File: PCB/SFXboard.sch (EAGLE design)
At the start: 19 parts, among them J1 AVR_SPI_PRG_6PTH, J2 TERMBLOCK4POS, J3 POWER_JACKPTH, Q1 16MHz, Q2 BSS138, Q3 BSS138, Q4 BSS138, U1 ATMEGA16U2-AU, X1 USBSMD

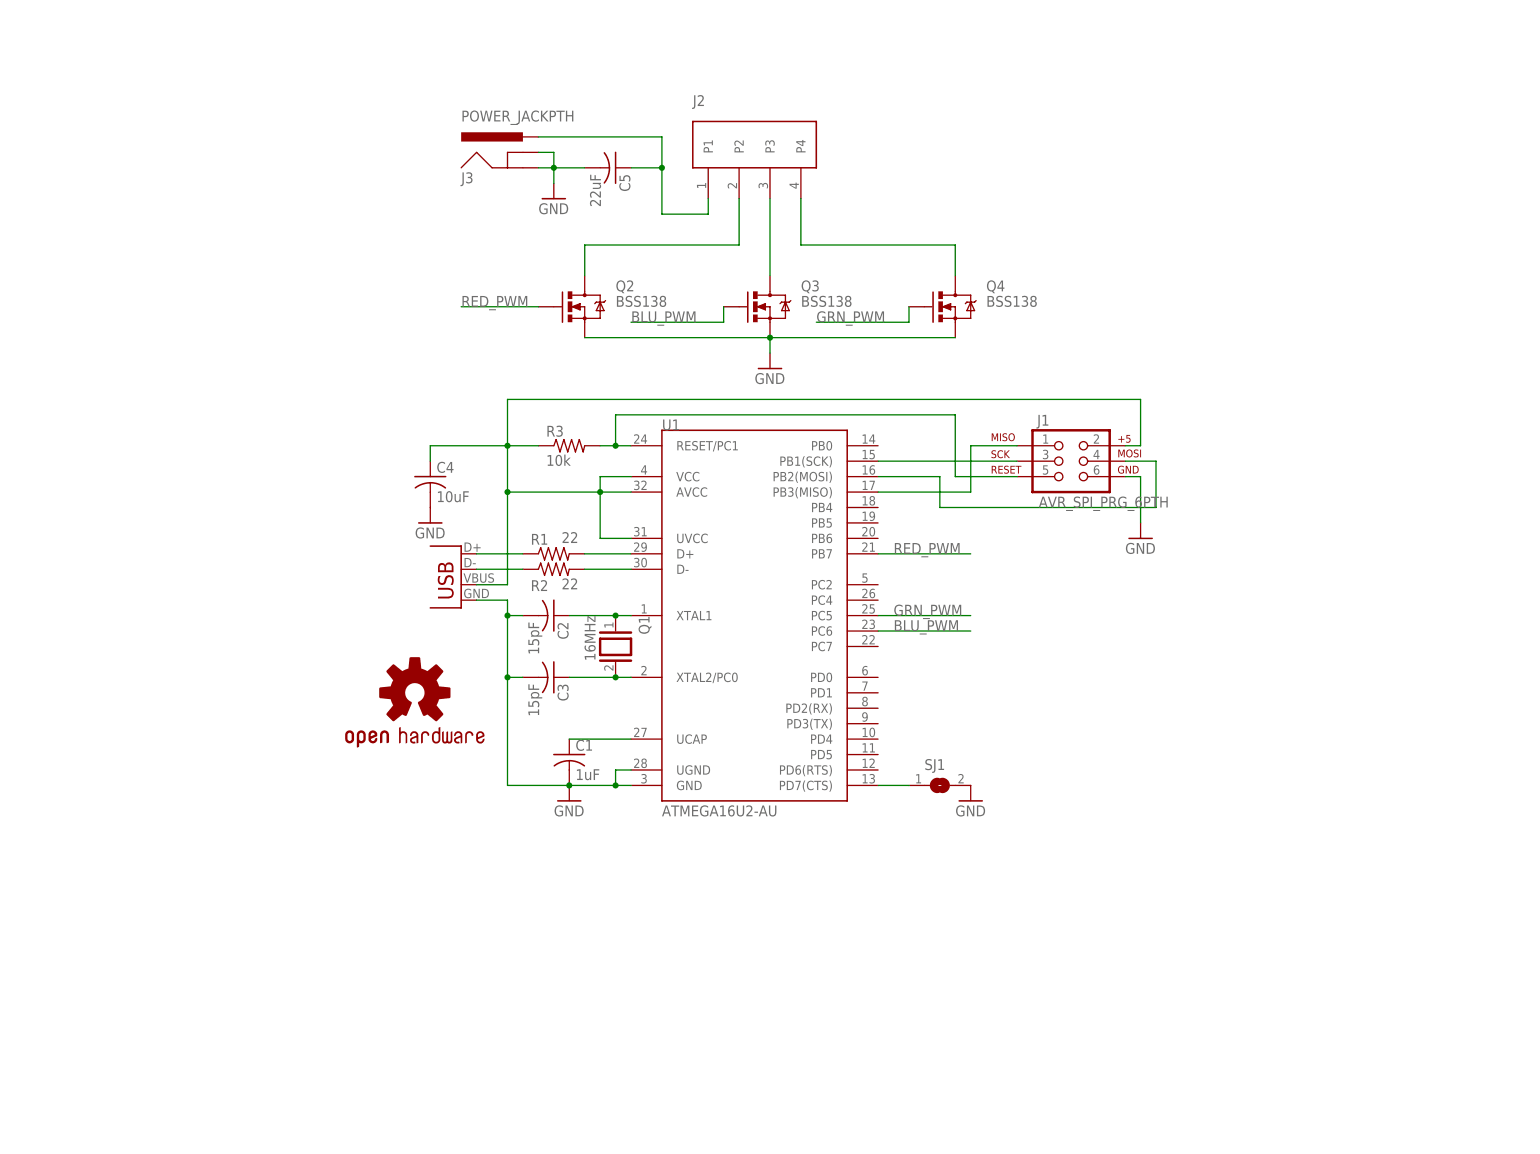
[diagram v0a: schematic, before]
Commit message: Circuit improvements, but not yet complete
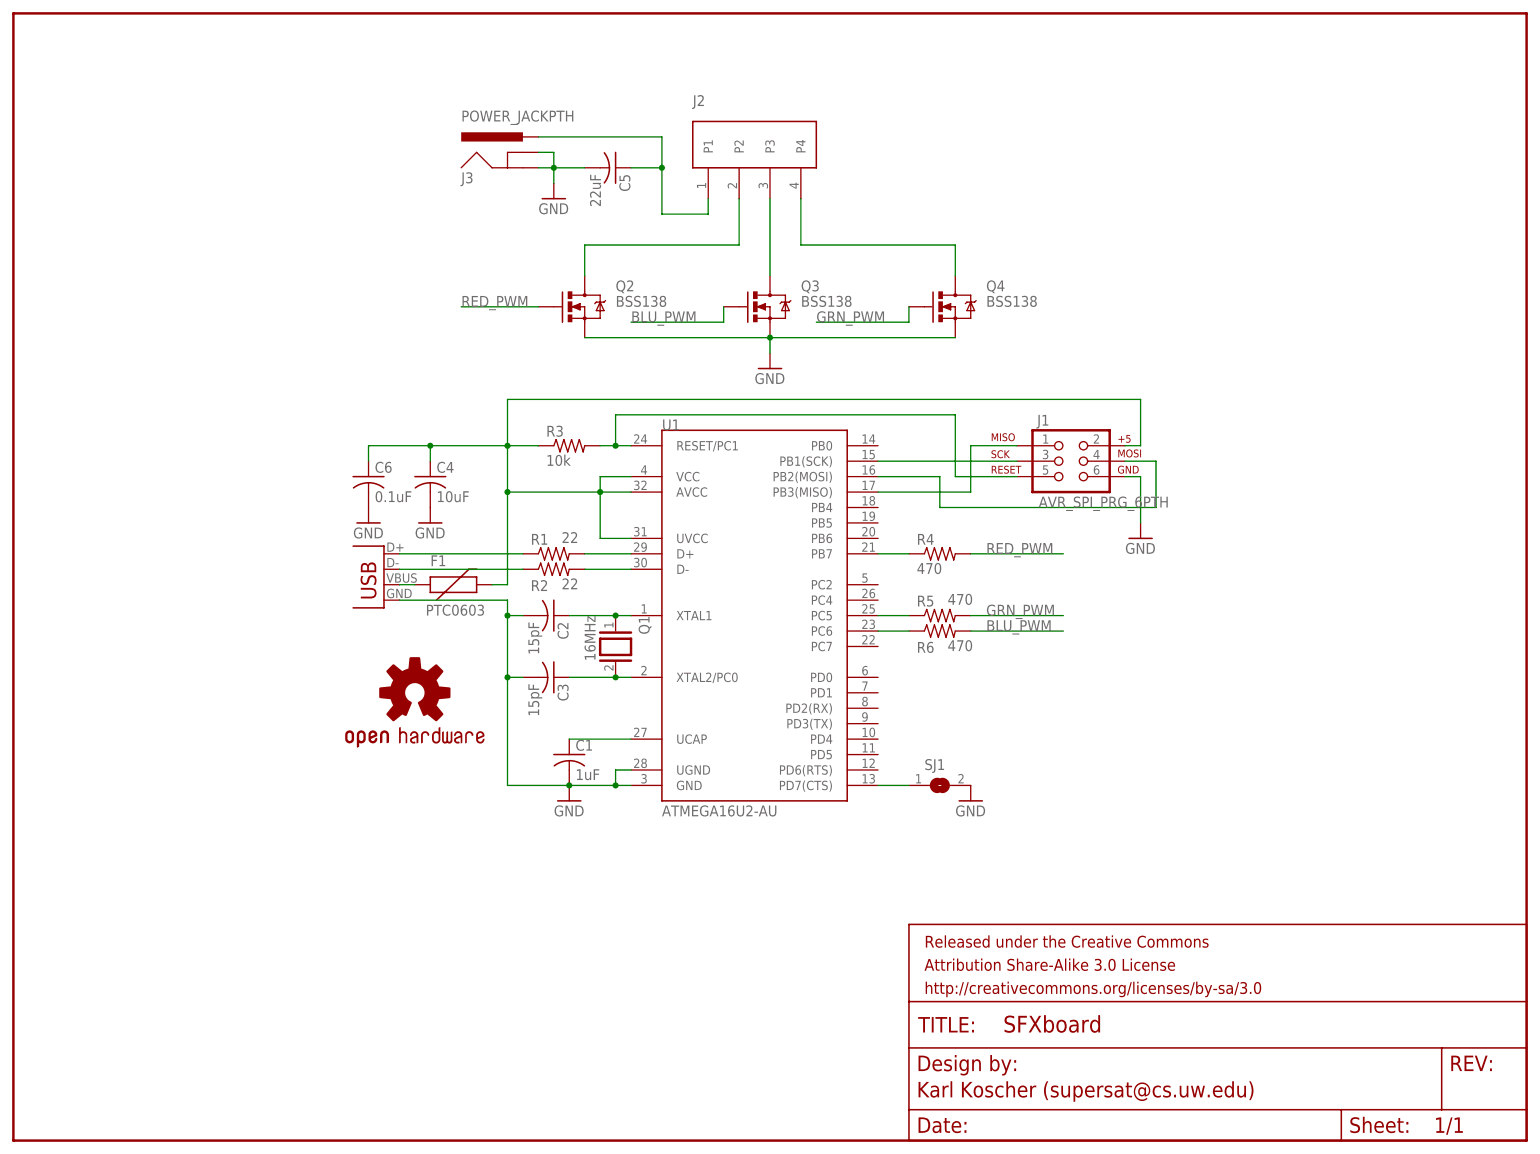
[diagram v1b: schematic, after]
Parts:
- added C6: 0.1uF, resistor:C-USC0402
- added F1: PTC0603, SparkFun-PowerIC:PTC0603
- added FRAME1: FRAME-LETTER, SparkFun-Aesthetics:FRAME-LETTER
- added R4, R5, R6: 470, resistor:R-US_R0805
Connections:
- new net B: R6.1, U1.PC6
- new net G: R5.1, U1.PC5
- new net N$18: C4.1, C6.1, F1.2, J1.2, R3.1, U1.AVCC, U1.UVCC, U1.VCC
- new net R: R4.1, U1.PB7
- net BLU_PWM: now also R6.2; no longer U1.PC6
- net GND: now also C6.2
- net GRN_PWM: now also R5.2; no longer U1.PC5
- net N$2: now also F1.1; no longer C4.1, J1.2, R3.1, U1.AVCC, U1.UVCC, U1.VCC
- net RED_PWM: now also R4.2; no longer U1.PB7
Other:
- note added: "Karl Koscher (supersat@cs.uw.edu)"
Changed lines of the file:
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@@
 <part name="SJ1" library="jumper" deviceset="SJ" device=""/>
 <part name="GND6" library="supply1" deviceset="GND" device=""/>
+<part name="C6" library="resistor" deviceset="C-US" device="C0402" value="0.1uF"/>
+<part name="GND7" library="supply1" deviceset="GND" device=""/>
+<part name="R4" library="resistor" deviceset="R-US_" device="R0805" value="470"/>
+<part name="R5" library="resistor" deviceset="R-US_" device="R0805" value="470"/>
+<part name="R6" library="resistor" deviceset="R-US_" device="R0805" value="470"/>
+<part name="FRAME1" library="SparkFun-Aesthetics" deviceset="FRAME-LETTER" device=""/>
+<part name="F1" library="SparkFun-PowerIC" deviceset="PTC" device="0603"/>
 </parts>
 <sheets>
 <sheet>
 <plain>
+<text x="26.67" y="-79.248" size="2.54" layer="94">Karl Koscher (supersat@cs.uw.edu)</text>
 </plain>
 <instances>
@@
 <instance part="C1" gate="G$1" x="-30.48" y="-22.86"/>
 <instance part="GND1" gate="1" x="-30.48" y="-30.48"/>
-<instance part="X1" gate="G$1" x="-48.26" y="2.54" rot="MR0"/>
+<instance part="X1" gate="G$1" x="-60.96" y="2.54" rot="MR0"/>
 <instance part="R1" gate="G$1" x="-33.02" y="10.16" smashed="yes">
 <attribute name="NAME" x="-36.83" y="11.6586" size="1.778" layer="95"/>
@@
 <instance part="SJ1" gate="1" x="30.48" y="-27.94"/>
 <instance part="GND6" gate="1" x="35.56" y="-30.48"/>
+<instance part="C6" gate="G$1" x="-63.5" y="22.86"/>
+<instance part="GND7" gate="1" x="-63.5" y="15.24"/>
+<instance part="R4" gate="G$1" x="30.48" y="10.16"/>
+<instance part="R5" gate="G$1" x="30.48" y="0" smashed="yes">
+<attribute name="NAME" x="26.67" y="1.4986" size="1.778" layer="95"/>
+<attribute name="VALUE" x="31.75" y="1.778" size="1.778" layer="96"/>
+</instance>
+<instance part="R6" gate="G$1" x="30.48" y="-2.54" smashed="yes">
+<attribute name="NAME" x="26.67" y="-6.1214" size="1.778" layer="95"/>
+<attribute name="VALUE" x="31.75" y="-5.842" size="1.778" layer="96"/>
+</instance>
+<instance part="FRAME1" gate="G$1" x="-121.92" y="-86.36"/>
+<instance part="FRAME1" gate="G$2" x="25.4" y="-86.36"/>
+<instance part="F1" gate="G$1" x="-50.8" y="5.08"/>
 </instances>
 <busses>
@@
 <wire x1="-40.64" y1="-10.16" x2="-40.64" y2="0" width="0.1524" layer="91"/>
 <wire x1="-40.64" y1="0" x2="-40.64" y2="2.54" width="0.1524" layer="91"/>
-<wire x1="-40.64" y1="2.54" x2="-45.72" y2="2.54" width="0.1524" layer="91"/>
+<wire x1="-40.64" y1="2.54" x2="-58.42" y2="2.54" width="0.1524" layer="91"/>
 <pinref part="C2" gate="G$1" pin="2"/>
 <wire x1="-38.1" y1="0" x2="-40.64" y2="0" width="0.1524" layer="91"/>
@@
 <pinref part="GND6" gate="1" pin="GND"/>
 </segment>
-</net>
-<net name="N$2" class="0">
-<segment>
-<pinref part="U1" gate="G$1" pin="VCC"/>
-<wire x1="-20.32" y1="22.86" x2="-25.4" y2="22.86" width="0.1524" layer="91"/>
-<wire x1="-25.4" y1="22.86" x2="-25.4" y2="20.32" width="0.1524" layer="91"/>
-<pinref part="U1" gate="G$1" pin="AVCC"/>
-<wire x1="-25.4" y1="20.32" x2="-20.32" y2="20.32" width="0.1524" layer="91"/>
-<pinref part="U1" gate="G$1" pin="UVCC"/>
-<wire x1="-20.32" y1="12.7" x2="-25.4" y2="12.7" width="0.1524" layer="91"/>
-<wire x1="-25.4" y1="20.32" x2="-25.4" y2="12.7" width="0.1524" layer="91"/>
-<pinref part="X1" gate="G$1" pin="VBUS"/>
-<wire x1="-45.72" y1="5.08" x2="-40.64" y2="5.08" width="0.1524" layer="91"/>
-<wire x1="-40.64" y1="5.08" x2="-40.64" y2="20.32" width="0.1524" layer="91"/>
-<wire x1="-40.64" y1="20.32" x2="-25.4" y2="20.32" width="0.1524" layer="91"/>
-<junction x="-25.4" y="20.32"/>
-<pinref part="R3" gate="G$1" pin="1"/>
-<wire x1="-35.56" y1="27.94" x2="-40.64" y2="27.94" width="0.1524" layer="91"/>
-<wire x1="-40.64" y1="27.94" x2="-40.64" y2="20.32" width="0.1524" layer="91"/>
-<junction x="-40.64" y="20.32"/>
-<pinref part="C4" gate="G$1" pin="1"/>
-<wire x1="-53.34" y1="25.4" x2="-53.34" y2="27.94" width="0.1524" layer="91"/>
-<wire x1="-53.34" y1="27.94" x2="-40.64" y2="27.94" width="0.1524" layer="91"/>
-<junction x="-40.64" y="27.94"/>
-<pinref part="J1" gate="G$1" pin="2"/>
-<wire x1="60.96" y1="27.94" x2="63.5" y2="27.94" width="0.1524" layer="91"/>
-<wire x1="63.5" y1="27.94" x2="63.5" y2="35.56" width="0.1524" layer="91"/>
-<wire x1="63.5" y1="35.56" x2="-40.64" y2="35.56" width="0.1524" layer="91"/>
-<wire x1="-40.64" y1="35.56" x2="-40.64" y2="27.94" width="0.1524" layer="91"/>
+<segment>
+<pinref part="C6" gate="G$1" pin="2"/>
+<pinref part="GND7" gate="1" pin="GND"/>
 </segment>
 </net>
@@
 <pinref part="X1" gate="G$1" pin="D+"/>
 <pinref part="R1" gate="G$1" pin="1"/>
-<wire x1="-45.72" y1="10.16" x2="-38.1" y2="10.16" width="0.1524" layer="91"/>
+<wire x1="-58.42" y1="10.16" x2="-38.1" y2="10.16" width="0.1524" layer="91"/>
 </segment>
 </net>
@@
 <pinref part="X1" gate="G$1" pin="D-"/>
 <pinref part="R2" gate="G$1" pin="1"/>
-<wire x1="-45.72" y1="7.62" x2="-38.1" y2="7.62" width="0.1524" layer="91"/>
+<wire x1="-58.42" y1="7.62" x2="-38.1" y2="7.62" width="0.1524" layer="91"/>
 </segment>
 </net>
@@
 <net name="RED_PWM" class="0">
 <segment>
-<pinref part="U1" gate="G$1" pin="PB7"/>
-<wire x1="20.32" y1="10.16" x2="35.56" y2="10.16" width="0.1524" layer="91"/>
-<label x="22.86" y="10.16" size="1.778" layer="95"/>
-</segment>
-<segment>
 <pinref part="Q2" gate="G$1" pin="G"/>
 <wire x1="-35.56" y1="50.8" x2="-48.26" y2="50.8" width="0.1524" layer="91"/>
 <label x="-48.26" y="50.8" size="1.778" layer="95"/>
+</segment>
+<segment>
+<pinref part="R4" gate="G$1" pin="2"/>
+<wire x1="35.56" y1="10.16" x2="50.8" y2="10.16" width="0.1524" layer="91"/>
+<label x="38.1" y="10.16" size="1.778" layer="95"/>
 </segment>
 </net>
@@
 </segment>
 <segment>
-<pinref part="U1" gate="G$1" pin="PC6"/>
-<wire x1="20.32" y1="-2.54" x2="35.56" y2="-2.54" width="0.1524" layer="91"/>
-<label x="22.86" y="-2.54" size="1.778" layer="95"/>
+<pinref part="R6" gate="G$1" pin="2"/>
+<wire x1="35.56" y1="-2.54" x2="50.8" y2="-2.54" width="0.1524" layer="91"/>
+<label x="38.1" y="-2.54" size="1.778" layer="95"/>
 </segment>
 </net>
@@
 </segment>
 <segment>
-<pinref part="U1" gate="G$1" pin="PC5"/>
-<wire x1="20.32" y1="0" x2="35.56" y2="0" width="0.1524" layer="91"/>
-<label x="22.86" y="0" size="1.778" layer="95"/>
+<pinref part="R5" gate="G$1" pin="2"/>
+<wire x1="35.56" y1="0" x2="50.8" y2="0" width="0.1524" layer="91"/>
+<label x="38.1" y="0" size="1.778" layer="95"/>
 </segment>
 </net>
@@
 </segment>
 </net>
+<net name="R" class="0">
+<segment>
+<pinref part="U1" gate="G$1" pin="PB7"/>
+<wire x1="20.32" y1="10.16" x2="25.4" y2="10.16" width="0.1524" layer="91"/>
+<pinref part="R4" gate="G$1" pin="1"/>
+</segment>
+</net>
+<net name="G" class="0">
+<segment>
+<pinref part="U1" gate="G$1" pin="PC5"/>
+<wire x1="20.32" y1="0" x2="25.4" y2="0" width="0.1524" layer="91"/>
+<pinref part="R5" gate="G$1" pin="1"/>
+</segment>
+</net>
+<net name="B" class="0">
+<segment>
+<pinref part="U1" gate="G$1" pin="PC6"/>
+<wire x1="20.32" y1="-2.54" x2="25.4" y2="-2.54" width="0.1524" layer="91"/>
+<pinref part="R6" gate="G$1" pin="1"/>
+</segment>
+</net>
+<net name="N$18" class="0">
+<segment>
+<pinref part="U1" gate="G$1" pin="VCC"/>
+<wire x1="-20.32" y1="22.86" x2="-25.4" y2="22.86" width="0.1524" layer="91"/>
+<wire x1="-25.4" y1="22.86" x2="-25.4" y2="20.32" width="0.1524" layer="91"/>
+<pinref part="U1" gate="G$1" pin="AVCC"/>
+<wire x1="-25.4" y1="20.32" x2="-20.32" y2="20.32" width="0.1524" layer="91"/>
+<pinref part="U1" gate="G$1" pin="UVCC"/>
+<wire x1="-20.32" y1="12.7" x2="-25.4" y2="12.7" width="0.1524" layer="91"/>
+<wire x1="-25.4" y1="20.32" x2="-25.4" y2="12.7" width="0.1524" layer="91"/>
+<wire x1="-40.64" y1="20.32" x2="-25.4" y2="20.32" width="0.1524" layer="91"/>
+<junction x="-25.4" y="20.32"/>
+<pinref part="R3" gate="G$1" pin="1"/>
+<wire x1="-35.56" y1="27.94" x2="-40.64" y2="27.94" width="0.1524" layer="91"/>
+<wire x1="-40.64" y1="27.94" x2="-40.64" y2="20.32" width="0.1524" layer="91"/>
+<pinref part="C4" gate="G$1" pin="1"/>
+<wire x1="-53.34" y1="25.4" x2="-53.34" y2="27.94" width="0.1524" layer="91"/>
+<wire x1="-53.34" y1="27.94" x2="-40.64" y2="27.94" width="0.1524" layer="91"/>
+<junction x="-40.64" y="27.94"/>
+<pinref part="J1" gate="G$1" pin="2"/>
+<wire x1="60.96" y1="27.94" x2="63.5" y2="27.94" width="0.1524" layer="91"/>
+<wire x1="63.5" y1="27.94" x2="63.5" y2="35.56" width="0.1524" layer="91"/>
+<wire x1="63.5" y1="35.56" x2="-40.64" y2="35.56" width="0.1524" layer="91"/>
+<wire x1="-40.64" y1="35.56" x2="-40.64" y2="27.94" width="0.1524" layer="91"/>
+<pinref part="C6" gate="G$1" pin="1"/>
+<wire x1="-53.34" y1="27.94" x2="-63.5" y2="27.94" width="0.1524" layer="91"/>
+<wire x1="-63.5" y1="27.94" x2="-63.5" y2="25.4" width="0.1524" layer="91"/>
+<junction x="-53.34" y="27.94"/>
+<wire x1="-40.64" y1="5.08" x2="-40.64" y2="20.32" width="0.1524" layer="91"/>
+<junction x="-40.64" y="20.32"/>
+<pinref part="F1" gate="G$1" pin="2"/>
+<wire x1="-40.64" y1="5.08" x2="-43.18" y2="5.08" width="0.1524" layer="91"/>
+</segment>
+</net>
+<net name="N$2" class="0">
+<segment>
+<pinref part="F1" gate="G$1" pin="1"/>
+<pinref part="X1" gate="G$1" pin="VBUS"/>
+<wire x1="-55.88" y1="5.08" x2="-58.42" y2="5.08" width="0.1524" layer="91"/>
+</segment>
+</net>
